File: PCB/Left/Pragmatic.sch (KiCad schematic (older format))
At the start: 75 parts, among them J1 Conn_02x07_Odd_Even, SW1 SW_Push, SW10 SW_Push, SW11 SW_Push, SW12 SW_Push, SW13 SW_Push, SW14 SW_Push, SW15 SW_Push, SW16 SW_Push, SW17 SW_Push, SW18 SW_Push, SW19 SW_Push, SW2 SW_Push, SW20 SW_Push, SW21 SW_Push, SW22 SW_Push, SW23 SW_Push, SW24 SW_Push, SW25 SW_Push, SW26 SW_Push, SW27 SW_Push, SW28 SW_Push, SW29 SW_Push, SW3 SW_Push, SW30 SW_Push, SW31 SW_Push, SW32 SW_Push, SW33 SW_Push, SW34 SW_Push, SW35 SW_Push, SW36 SW_Push, SW4 SW_Push, SW5 SW_Push, SW6 SW_Push, SW7 SW_Push, SW8 SW_Push, SW9 SW_Push

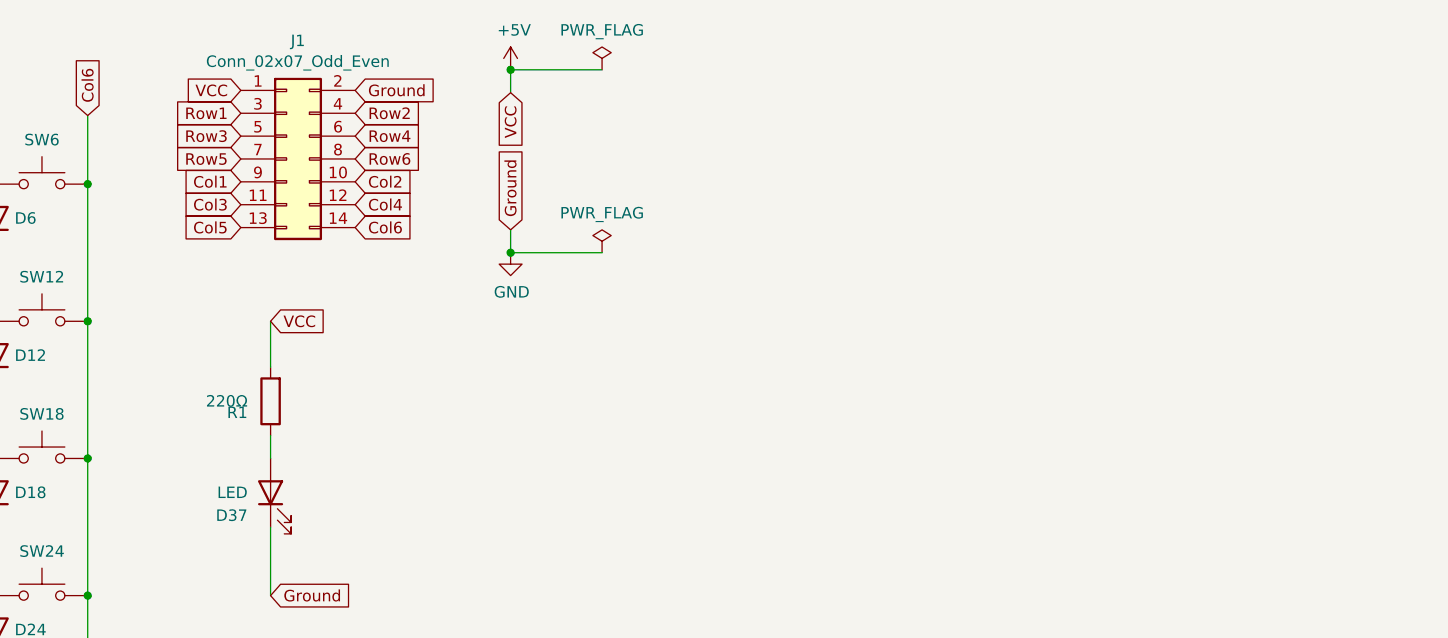
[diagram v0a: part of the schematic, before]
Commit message: double side design
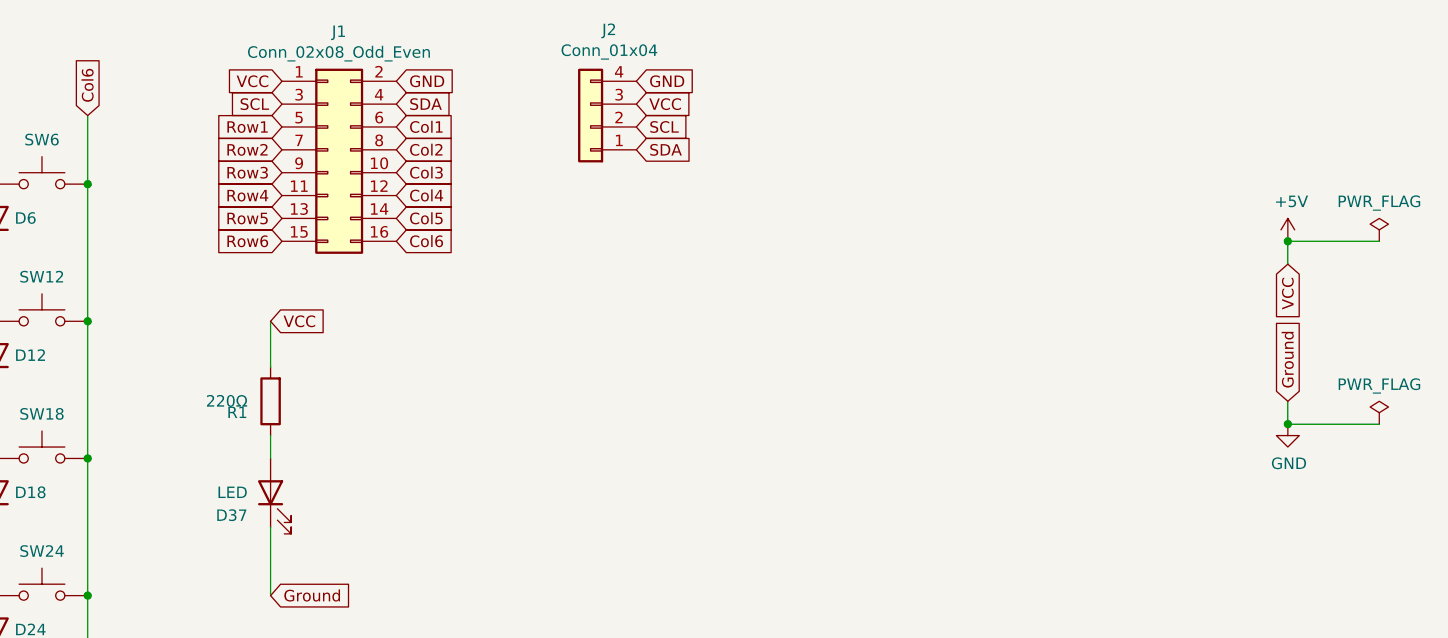
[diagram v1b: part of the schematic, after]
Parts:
- removed J1: Conn_02x07_Odd_Even, Connector_IDC:IDC-Header_2x07_P2.54mm_Vertical, symbol Connector_Generic:Conn_02x07_Odd_Even
- added J1: Conn_02x08_Odd_Even, Connector_IDC:IDC-Header_2x08_P2.54mm_Vertical, symbol Connector_Generic:Conn_02x08_Odd_Even
- added J2: Conn_01x04, kbd:OLED, symbol Connector_Generic:Conn_01x04
- D37: footprint LED_THT:LED_D3.0mm -> LED_SMD:LED_0805_2012Metric_Pad1.15x1.40mm_HandSolder
- R1: footprint Resistor_THT:R_Axial_DIN0207_L6.3mm_D2.5mm_P10.16mm_Horizontal -> Resistor_SMD:R_0805_2012Metric_Pad1.20x1.40mm_HandSolder
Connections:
- net +5V: now also J1.1 (Pin_1), J2.3 (Pin_3)
- net Col1: now also J1.6 (Pin_6)
- net Col2: now also J1.8 (Pin_8)
- net Col3: now also J1.10 (Pin_10)
- net Col4: now also J1.12 (Pin_12)
- net Col5: now also J1.14 (Pin_14)
- net Col6: now also J1.16 (Pin_16)
- net GND: now also J1.2 (Pin_2), J2.4 (Pin_4)
- net Row1: now also J1.5 (Pin_5)
- net Row2: now also J1.7 (Pin_7)
- net Row3: now also J1.9 (Pin_9)
- net Row4: now also J1.11 (Pin_11)
- net Row5: now also J1.13 (Pin_13)
- net Row6: now also J1.15 (Pin_15)
- new net SCL: J1.3 (Pin_3), J2.2 (Pin_2)
- new net SDA: J1.4 (Pin_4), J2.1 (Pin_1)
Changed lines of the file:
@@
 Comment4 ""
 $EndDescr
-Text GLabel 6750 3200 1    50   Input ~ 0
+Text GLabel 10150 3950 1    50   Input ~ 0
 Ground
 $Comp
 L power:+5V #PWR01
 U 1 1 6186CA9E
-P 6750 2500
-F 0 "#PWR01" H 6750 2350 50  0001 C CNN
-F 1 "+5V" H 6765 2673 50  0000 C CNN
-F 2 "" H 6750 2500 50  0001 C CNN
-F 3 "" H 6750 2500 50  0001 C CNN
-	1    6750 2500
-	1    0    0    -1
-$EndComp
-Text GLabel 6750 2600 3    50   Input ~ 0
+P 10150 3250
+F 0 "#PWR01" H 10150 3100 50  0001 C CNN
+F 1 "+5V" H 10165 3423 50  0000 C CNN
+F 2 "" H 10150 3250 50  0001 C CNN
+F 3 "" H 10150 3250 50  0001 C CNN
+	1    10150 3250
+	1    0    0    -1
+$EndComp
+Text GLabel 10150 3350 3    50   Input ~ 0
 VCC
 $Comp
 L power:GND #PWR02
 U 1 1 61895032
-P 6750 3300
-F 0 "#PWR02" H 6750 3050 50  0001 C CNN
-F 1 "GND" H 6755 3127 50  0000 C CNN
-F 2 "" H 6750 3300 50  0001 C CNN
-F 3 "" H 6750 3300 50  0001 C CNN
-	1    6750 3300
+P 10150 4050
+F 0 "#PWR02" H 10150 3800 50  0001 C CNN
+F 1 "GND" H 10155 3877 50  0000 C CNN
+F 2 "" H 10150 4050 50  0001 C CNN
+F 3 "" H 10150 4050 50  0001 C CNN
+	1    10150 4050
 	1    0    0    -1
 $EndComp
@@
 F 0 "D37" V 5600 4450 50  0000 L CNN
 F 1 "LED" V 5700 4450 50  0000 L CNN
-F 2 "LED_THT:LED_D3.0mm" H 5700 4350 50  0001 C CNN
+F 2 "LED_SMD:LED_0805_2012Metric_Pad1.15x1.40mm_HandSolder" H 5700 4350 50  0001 C CNN
 F 3 "~" H 5700 4350 50  0001 C CNN
 	1    5700 4350
@@
 F 0 "R1" H 5800 4000 50  0000 L CNN
 F 1 "220Ω" H 5800 3950 50  0000 L CNN
-F 2 "Resistor_THT:R_Axial_DIN0207_L6.3mm_D2.5mm_P10.16mm_Horizontal" V 5630 3950 50  0001 C CNN
+F 2 "Resistor_SMD:R_0805_2012Metric_Pad1.20x1.40mm_HandSolder" V 5630 3950 50  0001 C CNN
 F 3 "~" H 5700 3950 50  0001 C CNN
 	1    5700 3950
@@
 	0    -1   -1   0
 $EndComp
-$Comp
-L Connector_Generic:Conn_02x07_Odd_Even J1
-U 1 1 61867C1C
-P 5770 2890
-F 0 "J1" H 5820 3407 50  0000 C CNN
-F 1 "Conn_02x07_Odd_Even" H 5820 3316 50  0000 C CNN
-F 2 "Connector_IDC:IDC-Header_2x07_P2.54mm_Vertical" H 5770 2890 50  0001 C CNN
-F 3 "~" H 5770 2890 50  0001 C CNN
-	1    5770 2890
-	1    0    0    -1
-$EndComp
-Text GLabel 5570 2590 0    50   Input ~ 0
-VCC
-Text GLabel 5570 2690 0    50   Input ~ 0
-Row1
-Text GLabel 6070 2690 2    50   Input ~ 0
-Row2
-Text GLabel 5570 2790 0    50   Input ~ 0
-Row3
-Text GLabel 6070 2590 2    50   Input ~ 0
-Ground
-Text GLabel 5570 2990 0    50   Input ~ 0
-Col1
-Text GLabel 6070 2990 2    50   Input ~ 0
-Col2
-Text GLabel 6070 3190 2    50   Input ~ 0
-Col6
-Text GLabel 5570 3190 0    50   Input ~ 0
-Col5
-Text GLabel 6070 3090 2    50   Input ~ 0
-Col4
-Text GLabel 5570 3090 0    50   Input ~ 0
-Col3
-Text GLabel 6070 2790 2    50   Input ~ 0
-Row4
-Text GLabel 5570 2890 0    50   Input ~ 0
-Row5
-Text GLabel 6070 2890 2    50   Input ~ 0
-Row6
 $Comp
 L Switch:SW_Push SW8
@@
 	5700 4500 5700 4800
 Wire Wire Line
-	6750 2500 6750 2600
-Wire Wire Line
-	6750 3200 6750 3300
+	10150 3250 10150 3350
+Wire Wire Line
+	10150 3950 10150 4050
 Wire Wire Line
 	5700 4200 5700 4100
@@
 L power:PWR_FLAG #FLG0101
 U 1 1 6187BFDE
-P 7150 2500
-F 0 "#FLG0101" H 7150 2575 50  0001 C CNN
-F 1 "PWR_FLAG" H 7150 2673 50  0000 C CNN
-F 2 "" H 7150 2500 50  0001 C CNN
-F 3 "~" H 7150 2500 50  0001 C CNN
-	1    7150 2500
-	1    0    0    -1
-$EndComp
-Wire Wire Line
-	6750 2500 7150 2500
-Connection ~ 6750 2500
+P 10550 3250
+F 0 "#FLG0101" H 10550 3325 50  0001 C CNN
+F 1 "PWR_FLAG" H 10550 3423 50  0000 C CNN
+F 2 "" H 10550 3250 50  0001 C CNN
+F 3 "~" H 10550 3250 50  0001 C CNN
+	1    10550 3250
+	1    0    0    -1
+$EndComp
+Wire Wire Line
+	10150 3250 10550 3250
+Connection ~ 10150 3250
 $Comp
 L power:PWR_FLAG #FLG0102
 U 1 1 61881699
-P 7150 3300
-F 0 "#FLG0102" H 7150 3375 50  0001 C CNN
-F 1 "PWR_FLAG" H 7150 3473 50  0000 C CNN
-F 2 "" H 7150 3300 50  0001 C CNN
-F 3 "~" H 7150 3300 50  0001 C CNN
-	1    7150 3300
-	1    0    0    -1
-$EndComp
-Wire Wire Line
-	7150 3300 6750 3300
-Connection ~ 6750 3300
+P 10550 4050
+F 0 "#FLG0102" H 10550 4125 50  0001 C CNN
+F 1 "PWR_FLAG" H 10550 4223 50  0000 C CNN
+F 2 "" H 10550 4050 50  0001 C CNN
+F 3 "~" H 10550 4050 50  0001 C CNN
+	1    10550 4050
+	1    0    0    -1
+$EndComp
+Wire Wire Line
+	10550 4050 10150 4050
+Connection ~ 10150 4050
+$Comp
+L Connector_Generic:Conn_02x08_Odd_Even J1
+U 1 1 6194905D
+P 5950 2850
+F 0 "J1" H 6000 3367 50  0000 C CNN
+F 1 "Conn_02x08_Odd_Even" H 6000 3276 50  0000 C CNN
+F 2 "Connector_IDC:IDC-Header_2x08_P2.54mm_Vertical" H 5950 2850 50  0001 C CNN
+F 3 "~" H 5950 2850 50  0001 C CNN
+	1    5950 2850
+	1    0    0    -1
+$EndComp
+Text GLabel 5750 2550 0    50   Input ~ 0
+VCC
+Text GLabel 6250 2550 2    50   Input ~ 0
+GND
+Text GLabel 6250 2650 2    50   Input ~ 0
+SDA
+Text GLabel 5750 2650 0    50   Input ~ 0
+SCL
+Text GLabel 5750 2750 0    50   Input ~ 0
+Row1
+Text GLabel 5750 2850 0    50   Input ~ 0
+Row2
+Text GLabel 5750 2950 0    50   Input ~ 0
+Row3
+Text GLabel 5750 3050 0    50   Input ~ 0
+Row4
+Text GLabel 5750 3150 0    50   Input ~ 0
+Row5
+Text GLabel 5750 3250 0    50   Input ~ 0
+Row6
+Text GLabel 6250 2750 2    50   Input ~ 0
+Col1
+Text GLabel 6250 2850 2    50   Input ~ 0
+Col2
+Text GLabel 6250 2950 2    50   Input ~ 0
+Col3
+Text GLabel 6250 3050 2    50   Input ~ 0
+Col4
+Text GLabel 6250 3150 2    50   Input ~ 0
+Col5
+Text GLabel 6250 3250 2    50   Input ~ 0
+Col6
+$Comp
+L Connector_Generic:Conn_01x04 J2
+U 1 1 6195FBC7
+P 7100 2750
+F 0 "J2" H 7018 2325 50  0000 C CNN
+F 1 "Conn_01x04" H 7018 2416 50  0000 C CNN
+F 2 "kbd:OLED" H 7100 2750 50  0001 C CNN
+F 3 "~" H 7100 2750 50  0001 C CNN
+	1    7100 2750
+	-1   0    0    1
+$EndComp
+Text GLabel 7300 2550 2    50   Input ~ 0
+GND
+Text GLabel 7300 2750 2    50   Input ~ 0
+SCL
+Text GLabel 7300 2850 2    50   Input ~ 0
+SDA
+Text GLabel 7300 2650 2    50   Input ~ 0
+VCC
 $EndSCHEMATC
